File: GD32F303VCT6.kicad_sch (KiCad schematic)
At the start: 32 parts, among them SW1 SKRPACE010, U6 GD32F303VCT6, Y1 TAXM8M4RDBCCT2T, Y2 XKXGI-SUA-32.768K

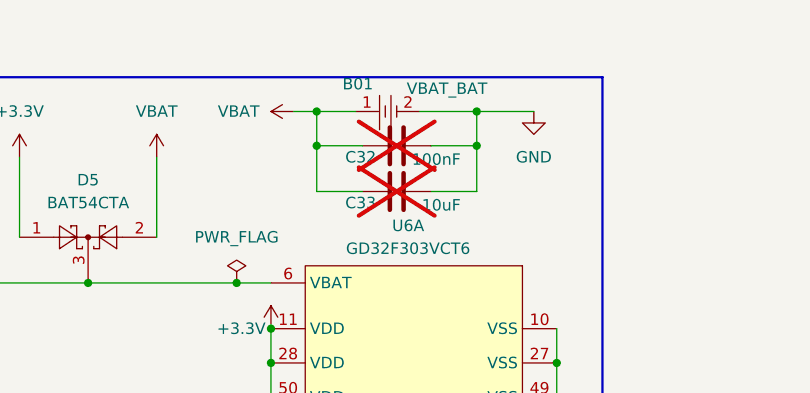
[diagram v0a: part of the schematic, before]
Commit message: 保存商业化布局优化前工程版本
- 保存当前PCB布局与走线调整
- 更新MCU核心页器件属性
- 记录后续商业板布局优化前的可回退检查点
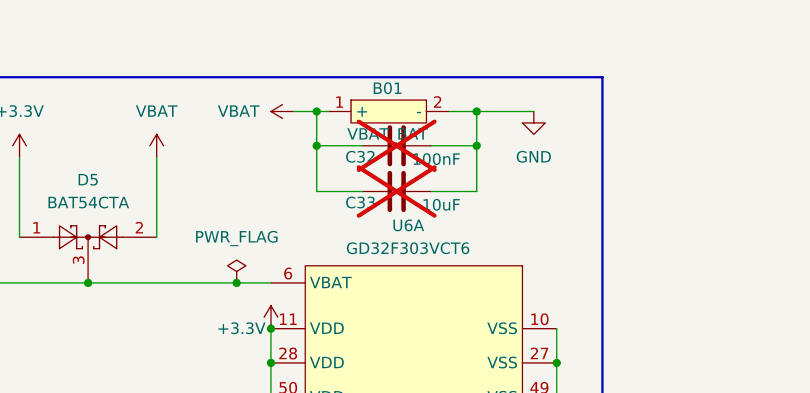
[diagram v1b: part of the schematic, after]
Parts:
- C32, C33: now left out of the parts list
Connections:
- net GND: no longer C32.2, C33.2, D5.2
- new net VBAT: C32.2, C33.2, D5.2
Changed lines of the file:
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@@
 	)
 	(junction
-		(at 76.2 29.21)
-		(diameter 0)
-		(color 0 0 0 0)
-	)
-	(junction
 		(at 71.12 60.96)
 		(diameter 0)
@@
 	)
 	(junction
-		(at 93.98 29.21)
-		(diameter 0)
-		(color 0 0 0 0)
-	)
-	(junction
 		(at 87.63 170.18)
 		(diameter 0)
@@
 	)
 	(junction
+		(at 93.98 29.21)
+		(diameter 0)
+		(color 0 0 0 0)
+	)
+	(junction
 		(at 59.055 113.03)
 		(diameter 0)
@@
 		(color 0 0 0 0)
 	)
+	(junction
+		(at 76.2 29.21)
+		(diameter 0)
+		(color 0 0 0 0)
+	)
 	(no_connect
 		(at 299.72 204.47)
@@
 		)
 	)
+	(wire
+		(pts
+			(xy 90.932 29.21) (xy 93.98 29.21)
+		)
+		(stroke
+			(width 0)
+			(type default)
+		)
+	)
 	(bus
 		(pts
@@
 	(wire
 		(pts
-			(xy 29.21 106.68) (xy 29.21 105.41)
+			(xy 76.2 29.21) (xy 77.47 29.21)
 		)
 		(stroke
@@
 	(wire
 		(pts
-			(xy 106.68 165.1) (xy 106.68 161.29)
+			(xy 29.21 106.68) (xy 29.21 105.41)
 		)
 		(stroke
@@
 	(wire
 		(pts
-			(xy 38.1 60.96) (xy 44.45 60.96)
+			(xy 106.68 165.1) (xy 106.68 161.29)
 		)
 		(stroke
@@
 	(wire
 		(pts
-			(xy 22.86 107.95) (xy 22.86 101.6)
+			(xy 38.1 60.96) (xy 44.45 60.96)
 		)
 		(stroke
@@
 	(wire
 		(pts
-			(xy 87.63 29.21) (xy 93.98 29.21)
+			(xy 22.86 107.95) (xy 22.86 101.6)
 		)
 		(stroke
@@
 	(wire
 		(pts
-			(xy 80.518 29.21) (xy 76.2 29.21)
-		)
-		(stroke
-			(width 0)
-			(type default)
-		)
-	)
-	(wire
-		(pts
 			(xy 93.98 29.21) (xy 93.98 33.02)
 		)
@@
 		(body_style 1)
 		(exclude_from_sim no)
-		(in_bom yes)
-		(on_board yes)
+		(in_bom no)
+		(on_board no)
 		(in_pos_files yes)
 		(dnp yes)
@@
 	(symbol
 		(lib_id "PZ254V-11-02P:VBAT_BAT")
-		(at 86.36 24.892 0)
+		(at 89.662 25.4 0)
 		(unit 1)
 		(body_style 1)
 		(exclude_from_sim no)
-		(in_bom yes)
+		(in_bom no)
 		(on_board yes)
 		(in_pos_files yes)
 		(dnp no)
 		(property "Reference" "B01"
-			(at 80.772 26.162 0)
+			(at 84.074 26.67 0)
 			(show_name no)
 			(do_not_autoplace no)
@@
 		)
 		(property "Value" "VBAT_BAT"
-			(at 90.678 26.67 0)
+			(at 84.074 31.75 0)
 			(show_name no)
 			(do_not_autoplace no)
@@
 			)
 		)
-		(property "Footprint" "Resistor_SMD:R_0603_1608Metric"
-			(at 86.36 24.892 0)
+		(property "Footprint" "Battery:BatteryHolder_Keystone_500"
+			(at 89.662 25.4 0)
 			(hide yes)
 			(show_name no)
@@
 		)
 		(property "Datasheet" ""
-			(at 86.36 24.892 0)
+			(at 89.662 25.4 0)
 			(hide yes)
 			(show_name no)
@@
 		)
 		(property "Description" ""
-			(at 86.36 24.892 0)
+			(at 89.662 25.4 0)
 			(hide yes)
 			(show_name no)
@@
 		(body_style 1)
 		(exclude_from_sim no)
-		(in_bom yes)
-		(on_board yes)
+		(in_bom no)
+		(on_board no)
 		(in_pos_files yes)
 		(dnp yes)
